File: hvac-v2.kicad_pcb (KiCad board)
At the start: 2 copper layers, 125 x 93 mm, 138 parts, among them J1 Anderson_two_redblack, J10 Conn_01x02, J11 Conn_01x03, J12 Conn_01x03, J13 Conn_01x03, J14 Conn_01x04, J2 Conn_01x04, J3 Conn_01x02, J4 Anderson_two_redblack_src, J5 Conn_01x03, J6 Conn_01x03, J7 Anderson_two_redblack_sink, J8 Anderson_two_redblack_sink, J9 Conn_01x02, Q1 AO3400A, Q2 AO3400A, Q3 AO3400A, SW1 SW_Push, SW2 Rotary_Encoder_Switch, U1 STM32F030C8Tx, U2 IFX007T, U3 IFX007T, U4 AMS1117-3.3, U5 DS18B20

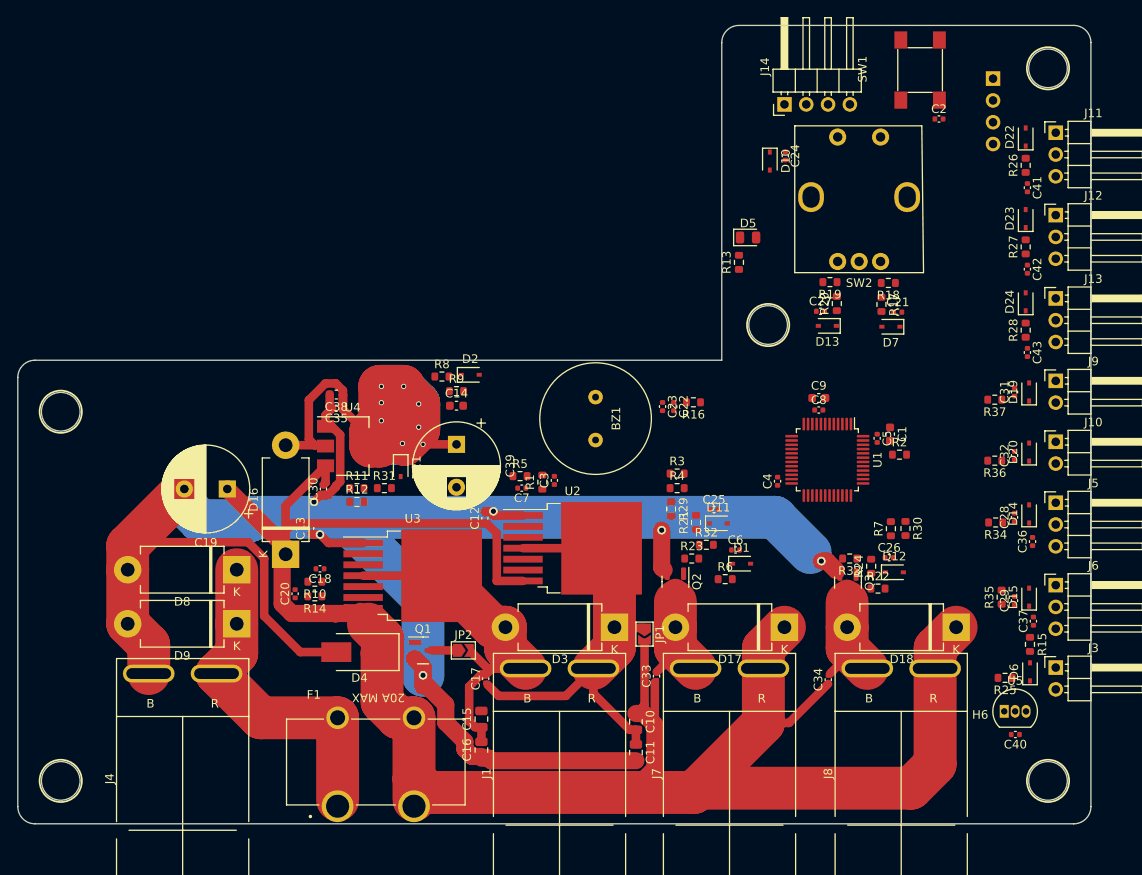
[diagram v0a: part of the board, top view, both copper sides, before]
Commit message: First pass at routing
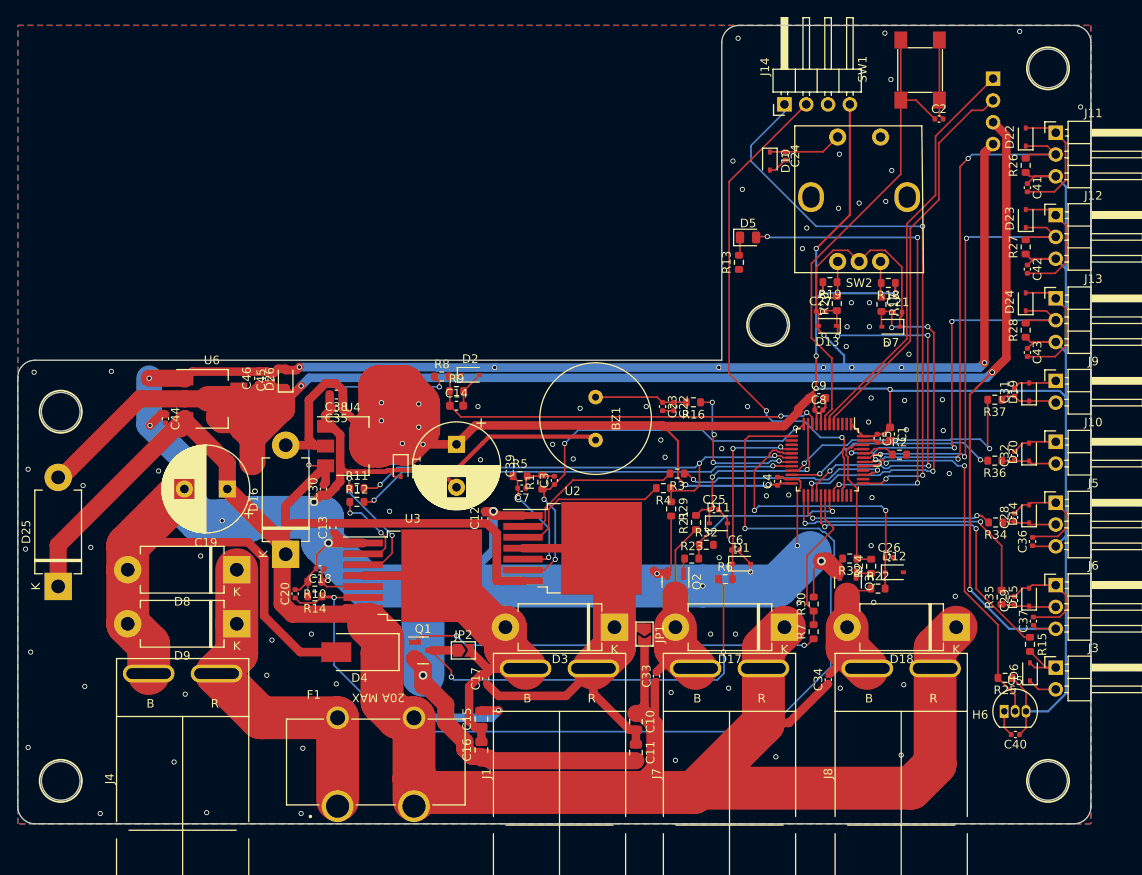
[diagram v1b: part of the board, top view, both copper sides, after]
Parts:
- removed R31: 110k, Resistor_SMD:R_0603_1608Metric
- added C44: 0.1uF, Capacitor_SMD:C_0402_1005Metric, F.Cu at (47.2, 104.8)
- added C45: 0.1uF, Capacitor_SMD:C_0402_1005Metric, F.Cu at (59.5, 100.3)
- added C46: 4.7uF, Capacitor_SMD:C_0603_1608Metric, F.Cu at (58.1, 100.1)
- added D25: D_Schottky, Diode_THT:D_DO-201AD_P12.70mm_Horizontal, F.Cu at (34.7, 124.3)
- added D26: TVS_5V, Diode_SMD:D_SOD-323, F.Cu at (61.2, 100.2)
- added U6: AMS1117-5.0, Package_TO_SOT_SMD:SOT-223-3_TabPin2, F.Cu at (52.6, 102.5)
- moved R7 15.0 mm to (122.7, 129.6)
- moved R30 13.9 mm to (122.7, 126.4), turned to 90 degrees
- moved C13 2.60 mm to (66.7, 117.5)
- moved R4 1.60 mm to (105.2, 112.9), turned to 180 degrees
- turned R3 to 180 degrees
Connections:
- C37 pad 1: VCC -> +5V
- J2 pad 3: VCC -> +5V
- J6 pad 3: VCC -> +5V
- U1 pad 14: /VBATT_DIV -> unconnected-(U1-Pad14)
- U1 pad 15: /PUMP_SENSE -> unconnected-(U1-Pad15)
- U1 pad 25: /SW_2 -> /SW_3
- U1 pad 26: /SW_3 -> /SW_2
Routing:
- net GND: track 232.2 -> 601.7 mm, vias 6 -> 97
- net VCC: track 78.8 -> 326.4 mm, vias 8 -> 14
- net +5V: track 0.00 -> 213.3 mm, vias 0 -> 4
- net /BRIDGE_SENSE_N: track 0.00 -> 123.9 mm, vias 0 -> 2
- net +BATT: track 240.1 -> 316.0 mm, vias 0 -> 3
- net /SWCLK: track 0.00 -> 67.7 mm, vias 0 -> 3
- net /TEMP_INSIDE: track 0.00 -> 64.9 mm, vias 0 -> 3
- net /BRIDGE_ENABLE: track 0.00 -> 59.5 mm, vias 0 -> 3
- net /SWDIO: track 0.00 -> 58.7 mm, vias 0 -> 2
- net /LED: track 0.00 -> 58.3 mm, vias 0 -> 4
- net /TEMP_OUTSIDE: track 0.00 -> 55.7 mm, vias 0 -> 3
- net /NRST: track 0.00 -> 55.3 mm
- net /BRIDGE_N: track 0.00 -> 51.6 mm, vias 0 -> 2
- net /BRIDGE_SENSE_P: track 0.00 -> 49.8 mm, vias 0 -> 4
- net /VBATT_DIV: track 0.00 -> 49.0 mm, vias 0 -> 2
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- added copper zone on B.Cu, net GND
- added copper zone on F.Cu, net GND
